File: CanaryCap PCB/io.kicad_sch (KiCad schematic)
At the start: 10 parts, among them J1 USB_C_Receptacle_USB2.0_16P

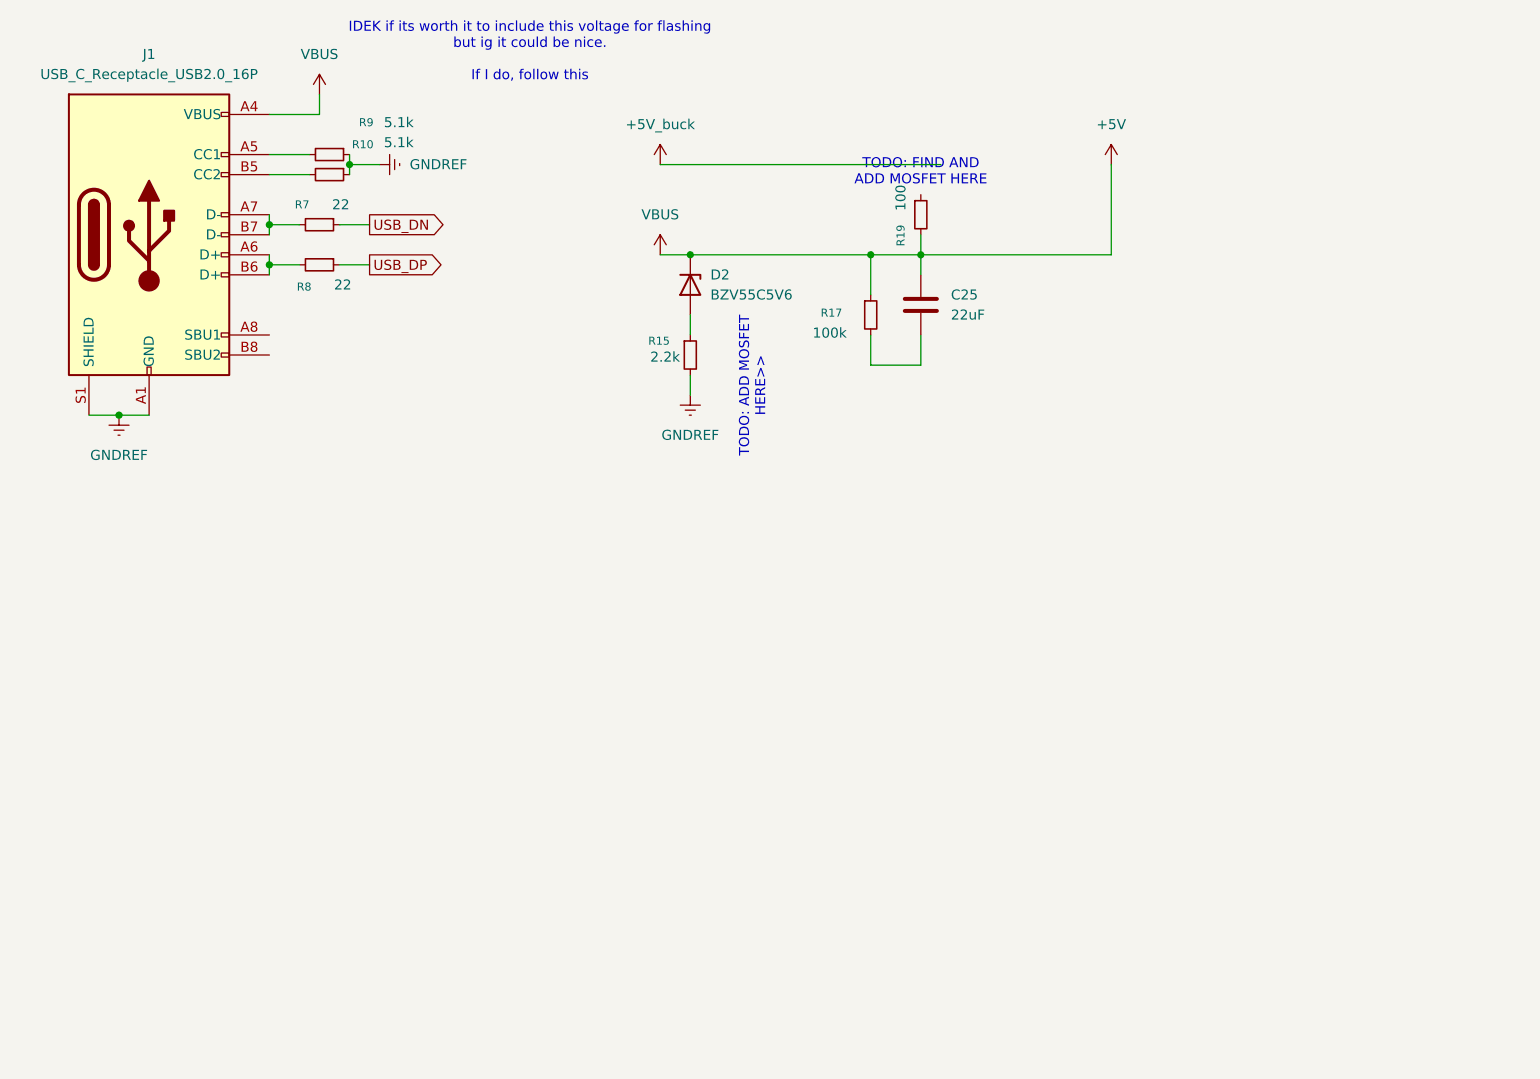
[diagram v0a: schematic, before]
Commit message: new changes
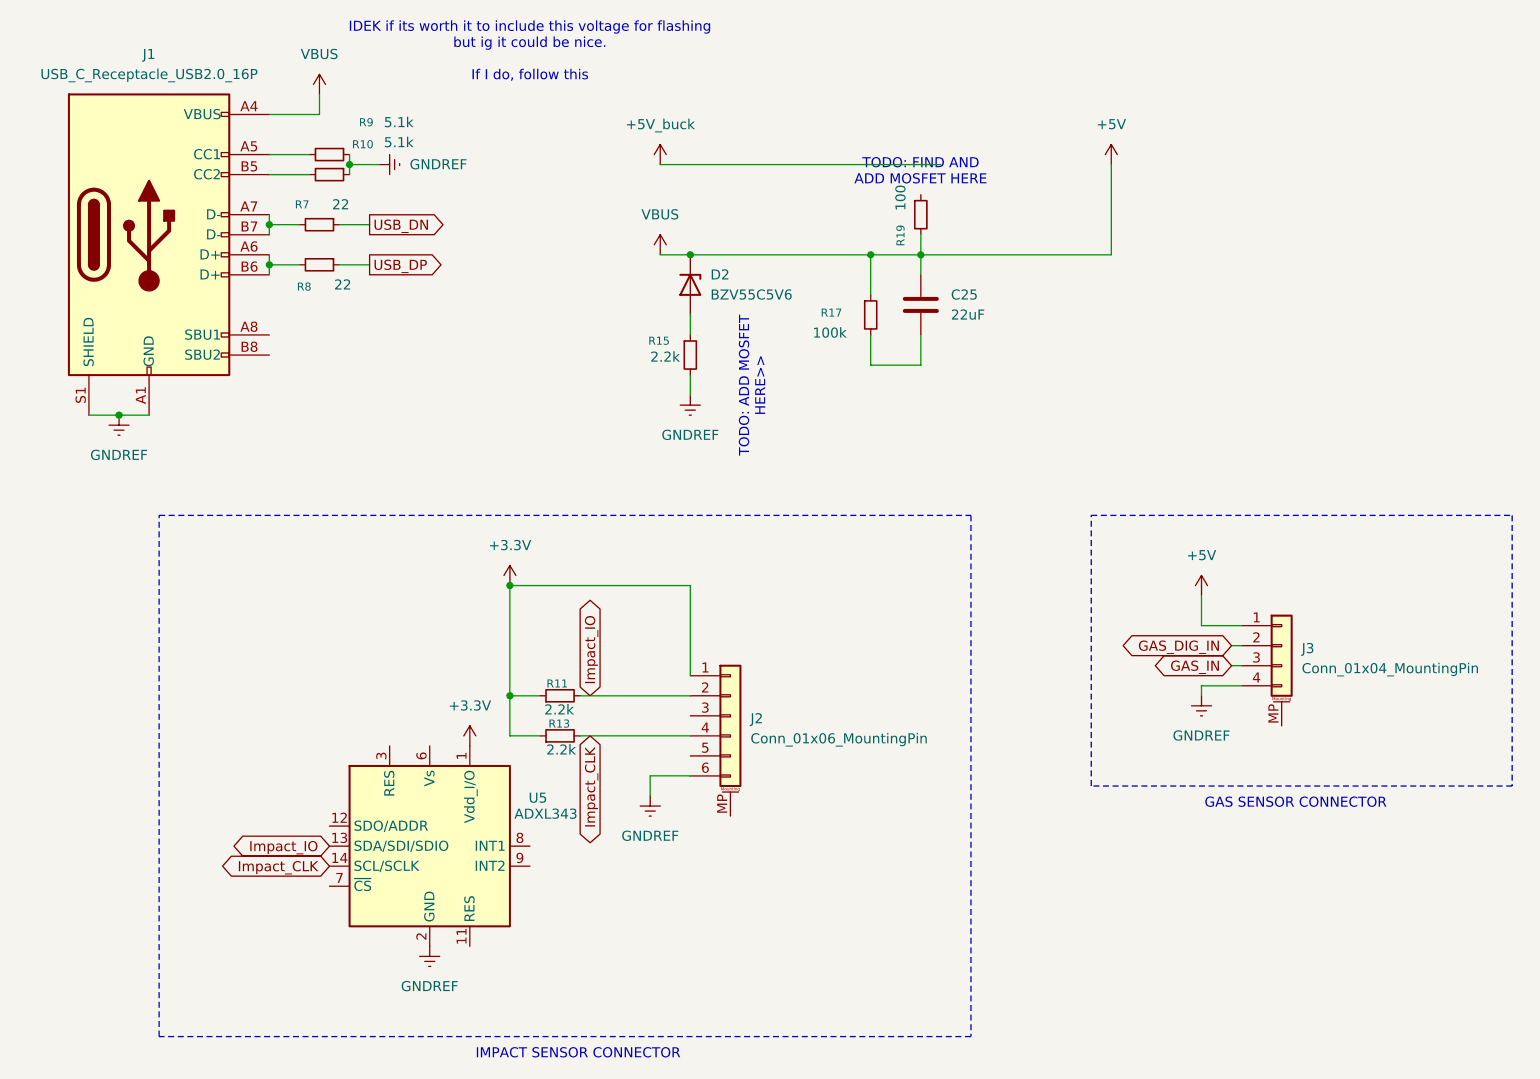
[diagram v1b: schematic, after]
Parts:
- added J2: Conn_01x06_MountingPin, symbol Connector_Generic_MountingPin:Conn_01x06_MountingPin
- added J3: Conn_01x04_MountingPin, symbol Connector_Generic_MountingPin:Conn_01x04_MountingPin
- added R11, R13: 2.2k, Resistor_SMD:R_0603_1608Metric_Pad0.98x0.95mm_HandSolder, symbol Device:R_Small
- added U5: ADXL343, Package_LGA:LGA-14_3x5mm_P0.8mm_LayoutBorder1x6y, symbol Sensor_Motion:ADXL343
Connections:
- net +5V: now also J3.1 (Pin_1)
- net GNDREF: now also J2.6 (Pin_6), J3.4 (Pin_4), U5.2 (GND), U5.4 (GND), U5.5 (GND)
- new net +3.3V: J2.1 (Pin_1), R11.1, R13.1, U5.1 (Vdd_I/O)
- new net GAS_DIG_IN: J3.2 (Pin_2)
- new net GAS_IN: J3.3 (Pin_3)
- new net Impact_CLK: J2.4 (Pin_4), R13.2, U5.14 (SCL/SCLK)
- new net Impact_IO: J2.2 (Pin_2), R11.2, U5.13 (SDA/SDI/SDIO)
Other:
- note added: "GAS SENSOR CONNECTOR"
- note added: "IMPACT SENSOR CONNECTOR"
